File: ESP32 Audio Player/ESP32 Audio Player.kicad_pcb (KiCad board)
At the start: 2 copper layers, 75.5 x 72 mm, 8 parts, among them SW1 SW_Push, SW2 SW_Push, SW3 SW_Push, U1 TP4056, U2 OLED

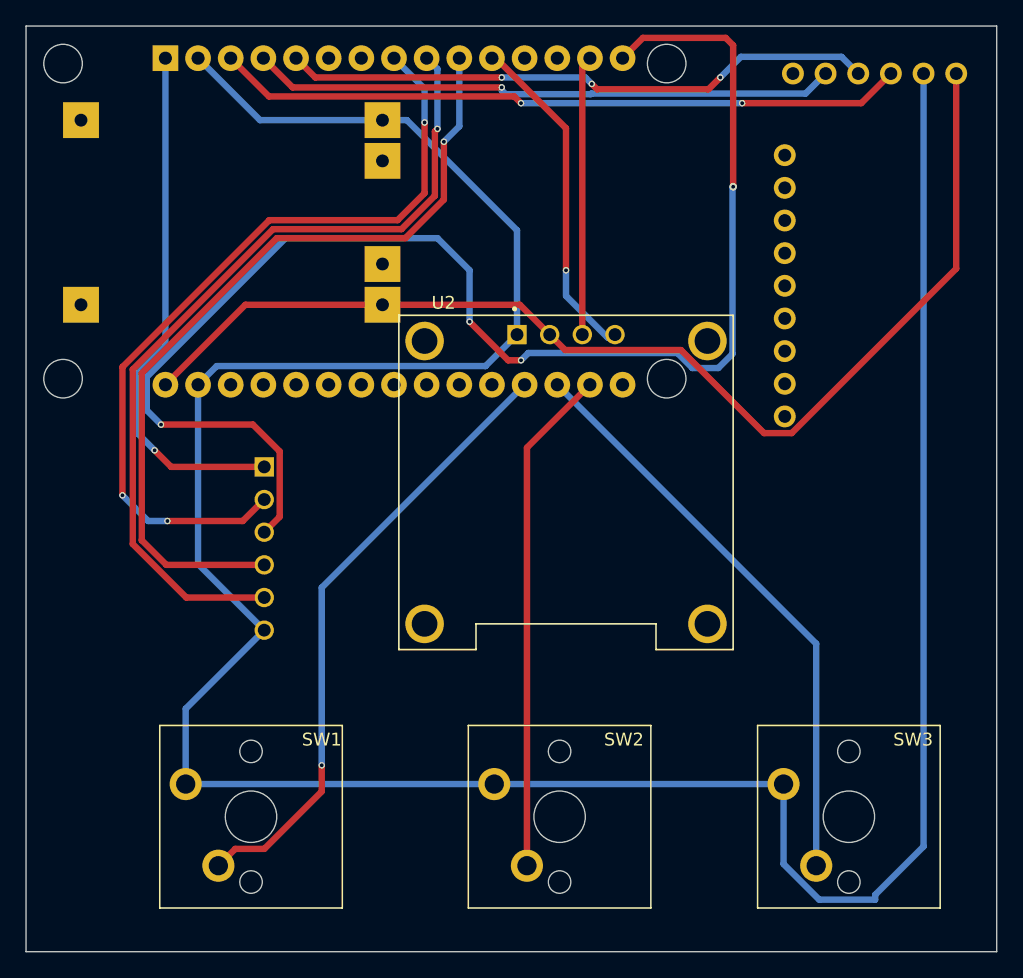
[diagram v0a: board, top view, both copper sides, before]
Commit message: Added gerber files
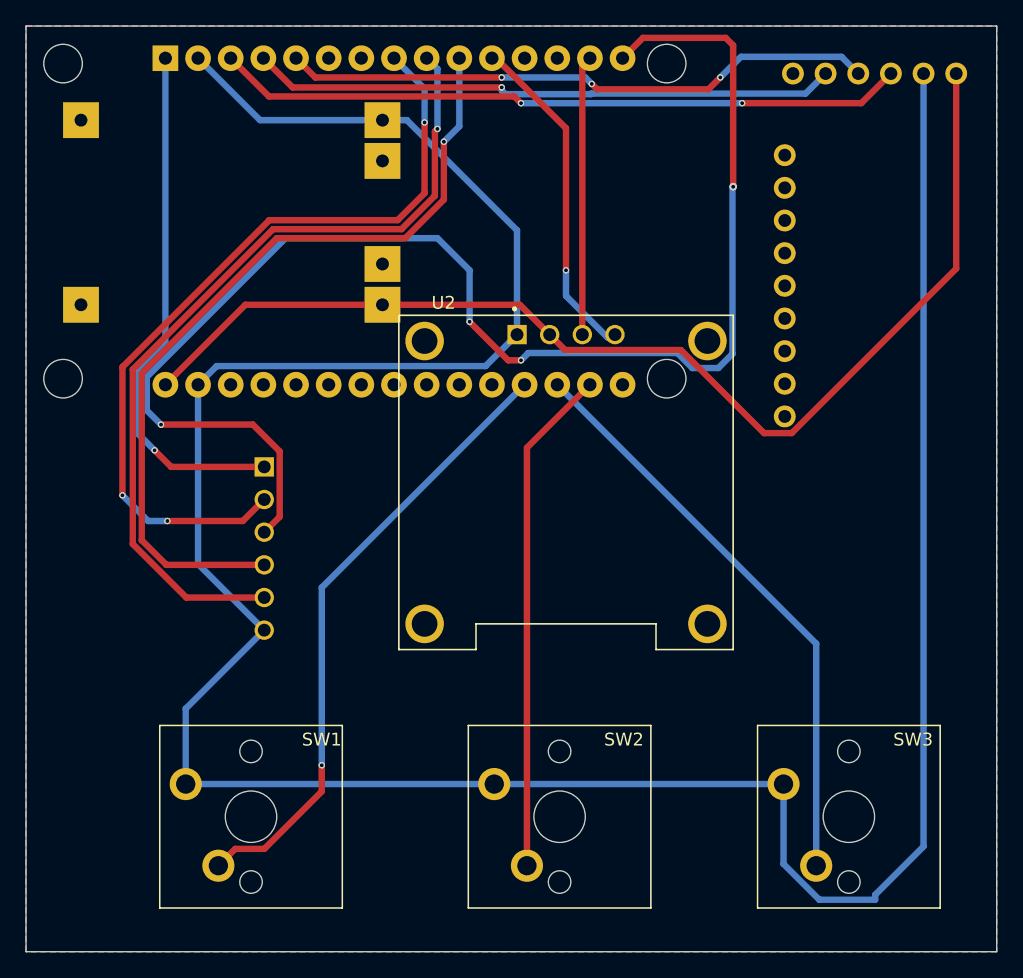
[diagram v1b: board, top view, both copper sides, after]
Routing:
- added copper zone on B.Cu, net GND
- added copper zone on F.Cu, net GND
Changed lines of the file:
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@@
 			(outputformat 1)
 			(mirror no)
-			(drillshape 1)
+			(drillshape 0)
 			(scaleselection 1)
-			(outputdirectory "")
+			(outputdirectory "ESP32 Audio Player/")
 		)
 	)
@@
 	)
 	(segment
-		(start 73 68)
-		(end 74.5 68)
+		(start 94.5 37)
+		(end 94.5 34.38)
 		(width 0.5)
 		(layer "B.Cu")
@@
 	)
 	(segment
-		(start 94.5 37)
-		(end 94.5 34.38)
+		(start 73 68)
+		(end 71 66)
 		(width 0.5)
 		(layer "B.Cu")
@@
 	)
 	(segment
-		(start 71 66)
+		(start 74.5 68)
 		(end 73 68)
 		(width 0.5)
@@
 		(net "Net-(MCU1-D18)")
 	)
+	(zone
+		(net "GND")
+		(layer "F.Cu")
+		(hatch edge 0.5)
+		(connect_pads
+			(clearance 0.5)
+		)
+		(min_thickness 0.25)
+		(fill yes
+			(thermal_gap 0.5)
+			(thermal_bridge_width 0.5)
+			(island_removal_mode 0)
+		)
+		(polygon
+			(pts
+				(xy 63.5 29.5) (xy 139 29.5) (xy 139 101.5) (xy 63.5 101.5)
+			)
+		)
+	)
+	(zone
+		(net "GND")
+		(layer "B.Cu")
+		(hatch edge 0.5)
+		(priority 1)
+		(connect_pads
+			(clearance 0.5)
+		)
+		(min_thickness 0.25)
+		(fill yes
+			(thermal_gap 0.5)
+			(thermal_bridge_width 0.5)
+			(island_removal_mode 0)
+		)
+		(polygon
+			(pts
+				(xy 63.5 29.5) (xy 139 29.5) (xy 139 101.5) (xy 63.5 101.5)
+			)
+		)
+	)
 	(embedded_fonts no)
